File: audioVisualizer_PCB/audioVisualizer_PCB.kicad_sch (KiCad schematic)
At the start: 42 parts, among them J1 USB_C_16P, J2 SWD_DEBUG, J3 SPI_LED_MATRIX, SW1 SW_Push, U1 AMS1117-3.3, U2 STM32F401RETx, Y1 ASE-25MHz

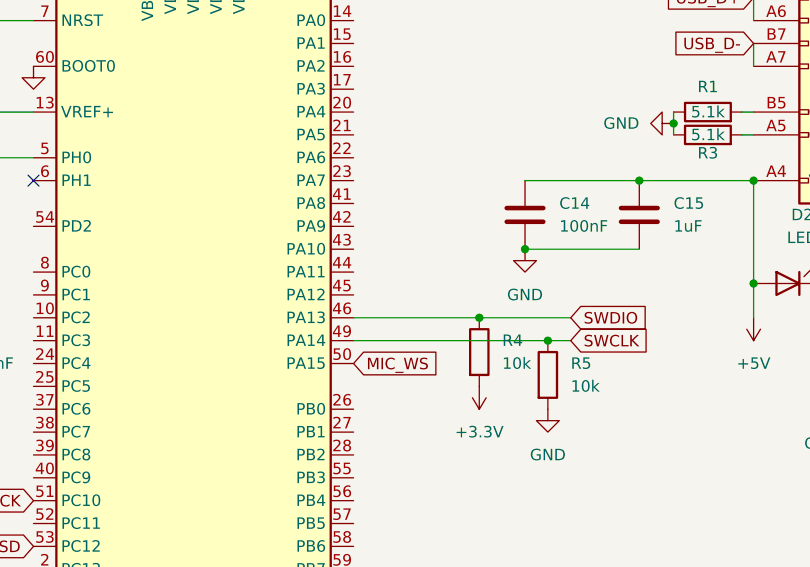
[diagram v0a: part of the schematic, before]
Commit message: connected the usb, incase it worked
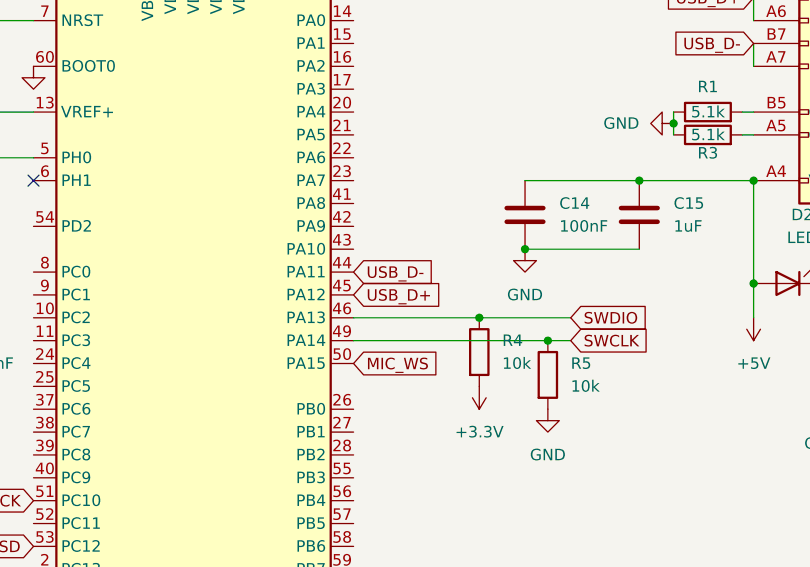
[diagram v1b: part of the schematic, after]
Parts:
- R1, R3: footprint Resistor_SMD:R_0805_2012Metric -> Resistor_SMD:R_1206_3216Metric
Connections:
- net USB_D+: now also U2.45 (PA12)
- net USB_D-: now also U2.44 (PA11)
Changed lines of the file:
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@@
 		)
 	)
+	(global_label "USB_D+"
+		(shape input)
+		(at 209.55 71.12 0)
+		(fields_autoplaced yes)
+		(effects
+			(font
+				(size 1.27 1.27)
+			)
+			(justify left)
+		)
+		(property "Intersheetrefs" "${INTERSHEET_REFS}"
+			(at 220.1552 71.12 0)
+			(hide yes)
+			(show_name no)
+			(do_not_autoplace no)
+			(effects
+				(font
+					(size 1.27 1.27)
+				)
+				(justify left)
+			)
+		)
+	)
 	(global_label "MIC_WS"
 		(shape input)
@@
 		)
 	)
+	(global_label "USB_D-"
+		(shape input)
+		(at 209.55 68.58 0)
+		(fields_autoplaced yes)
+		(effects
+			(font
+				(size 1.27 1.27)
+			)
+			(justify left)
+		)
+		(property "Intersheetrefs" "${INTERSHEET_REFS}"
+			(at 220.1552 68.58 0)
+			(hide yes)
+			(show_name no)
+			(do_not_autoplace no)
+			(effects
+				(font
+					(size 1.27 1.27)
+				)
+				(justify left)
+			)
+		)
+	)
 	(global_label "SWCLK"
 		(shape input)
@@
 			)
 		)
-		(property "Footprint" "Resistor_SMD:R_0805_2012Metric"
+		(property "Footprint" "Resistor_SMD:R_1206_3216Metric"
 			(at 248.92 52.578 90)
 			(hide yes)
@@
 			)
 		)
-		(property "Footprint" "Resistor_SMD:R_0805_2012Metric"
+		(property "Footprint" "Resistor_SMD:R_1206_3216Metric"
 			(at 248.92 55.118 90)
 			(hide yes)
